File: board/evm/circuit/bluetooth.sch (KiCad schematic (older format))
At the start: 1 part

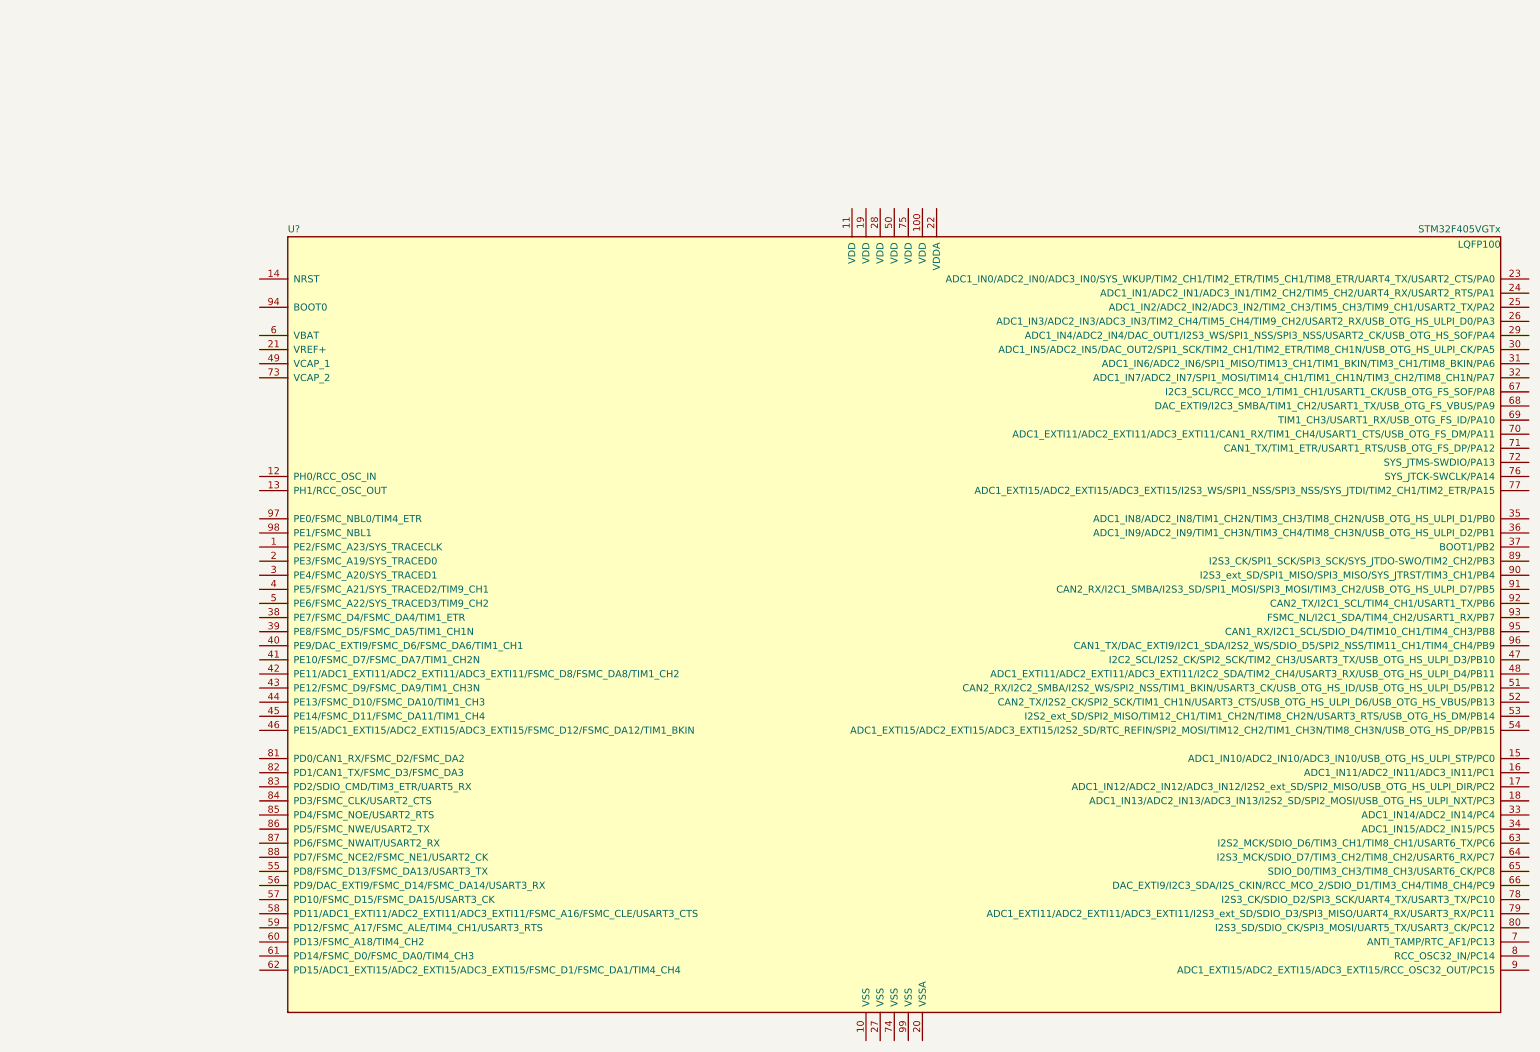
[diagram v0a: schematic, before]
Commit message: add lots of ICs
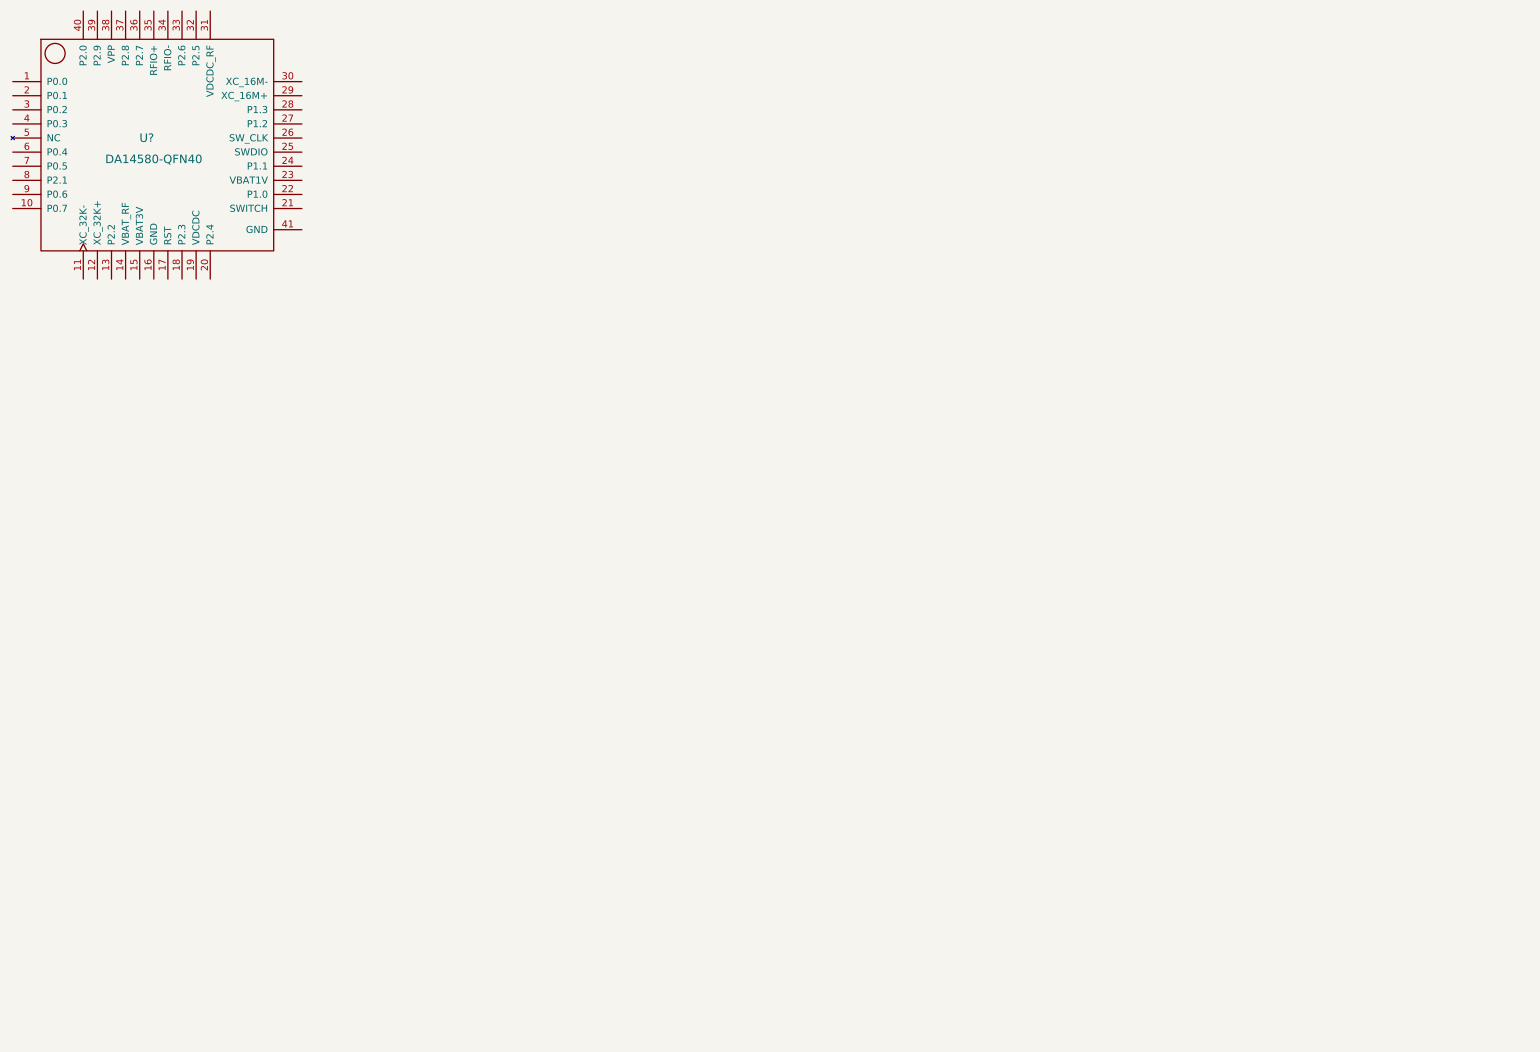
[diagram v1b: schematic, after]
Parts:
- removed U?: STM32F405VGTx, LQFP100, symbol STM32F405VGTx
- added U?: DA14580-QFN40, symbol DA14580-QFN40
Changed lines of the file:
@@
 EELAYER 25 0
 EELAYER END
-$Descr A2 23386 16535
+$Descr A4 11693 8268
 encoding utf-8
-Sheet 2 8
+Sheet 6 8
 Title ""
 Date ""
@@
 $EndDescr
 $Comp
-L STM32F405VGTx U?
-U 1 1 5753F449
-P 9650 6400
-F 0 "U?" H 5350 9225 50  0000 L BNN
-F 1 "STM32F405VGTx" H 13950 9225 50  0000 R BNN
-F 2 "LQFP100" H 13950 9175 50  0000 R TNN
-F 3 "" H 9650 6400 50  0000 C CNN
-	1    9650 6400
+L DA14580-QFN40 U?
+U 1 1 575491AD
+P 4450 2950
+F 0 "U?" H 4350 3000 60  0000 C CNN
+F 1 "DA14580-QFN40" H 4400 2850 60  0000 C CNN
+F 2 "" H 4350 3000 60  0000 C CNN
+F 3 "" H 4350 3000 60  0000 C CNN
+	1    4450 2950
 	1    0    0    -1
 $EndComp
